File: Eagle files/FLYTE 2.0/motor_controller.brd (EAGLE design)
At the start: 160 x 100 mm, 21 parts, among them J1 XT60PW-F

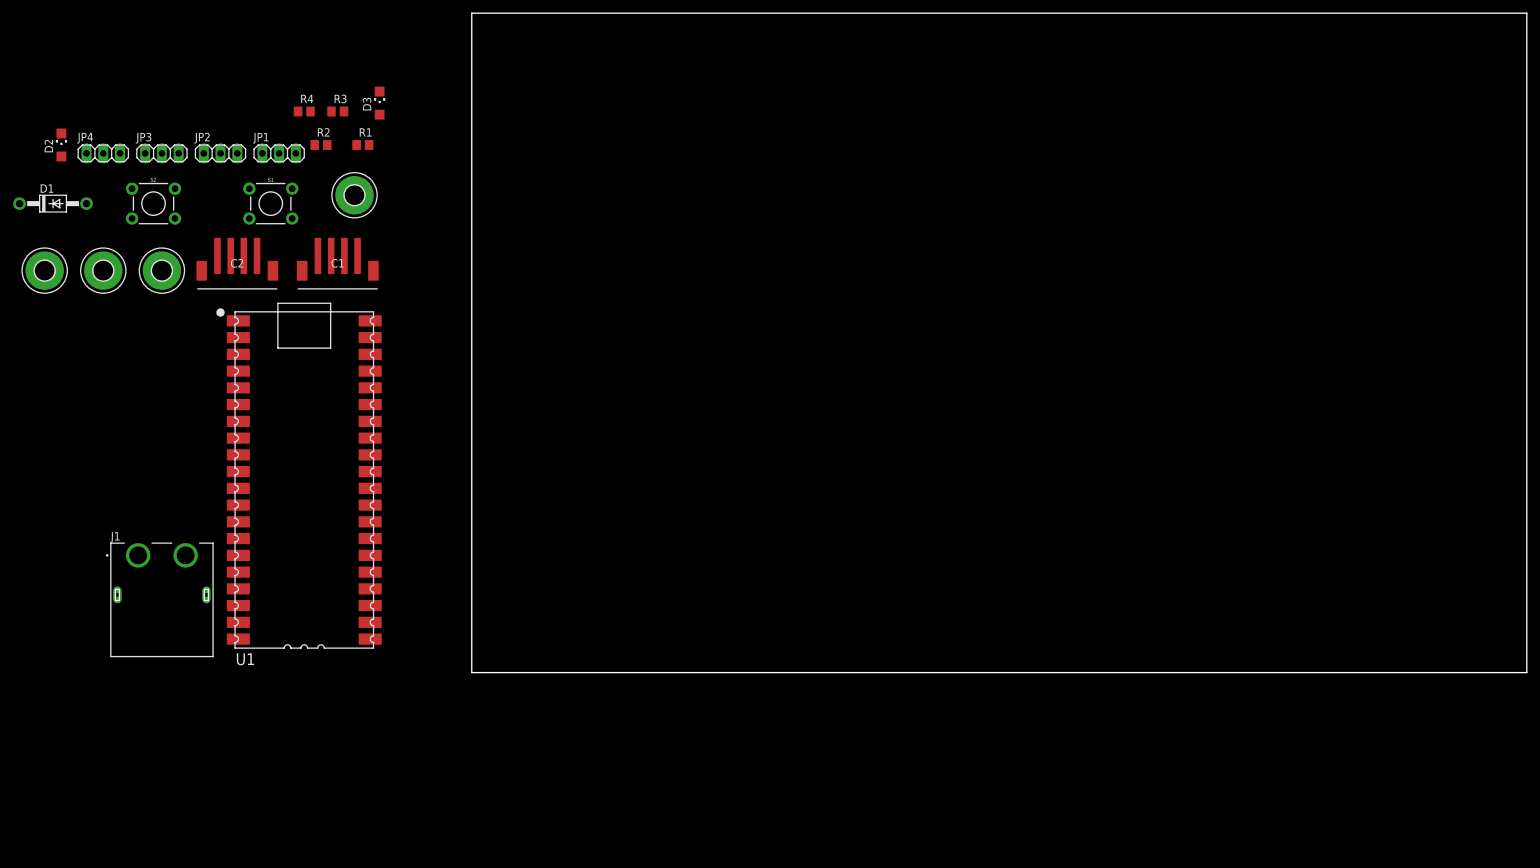
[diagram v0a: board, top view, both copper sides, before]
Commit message: Finish motor controller
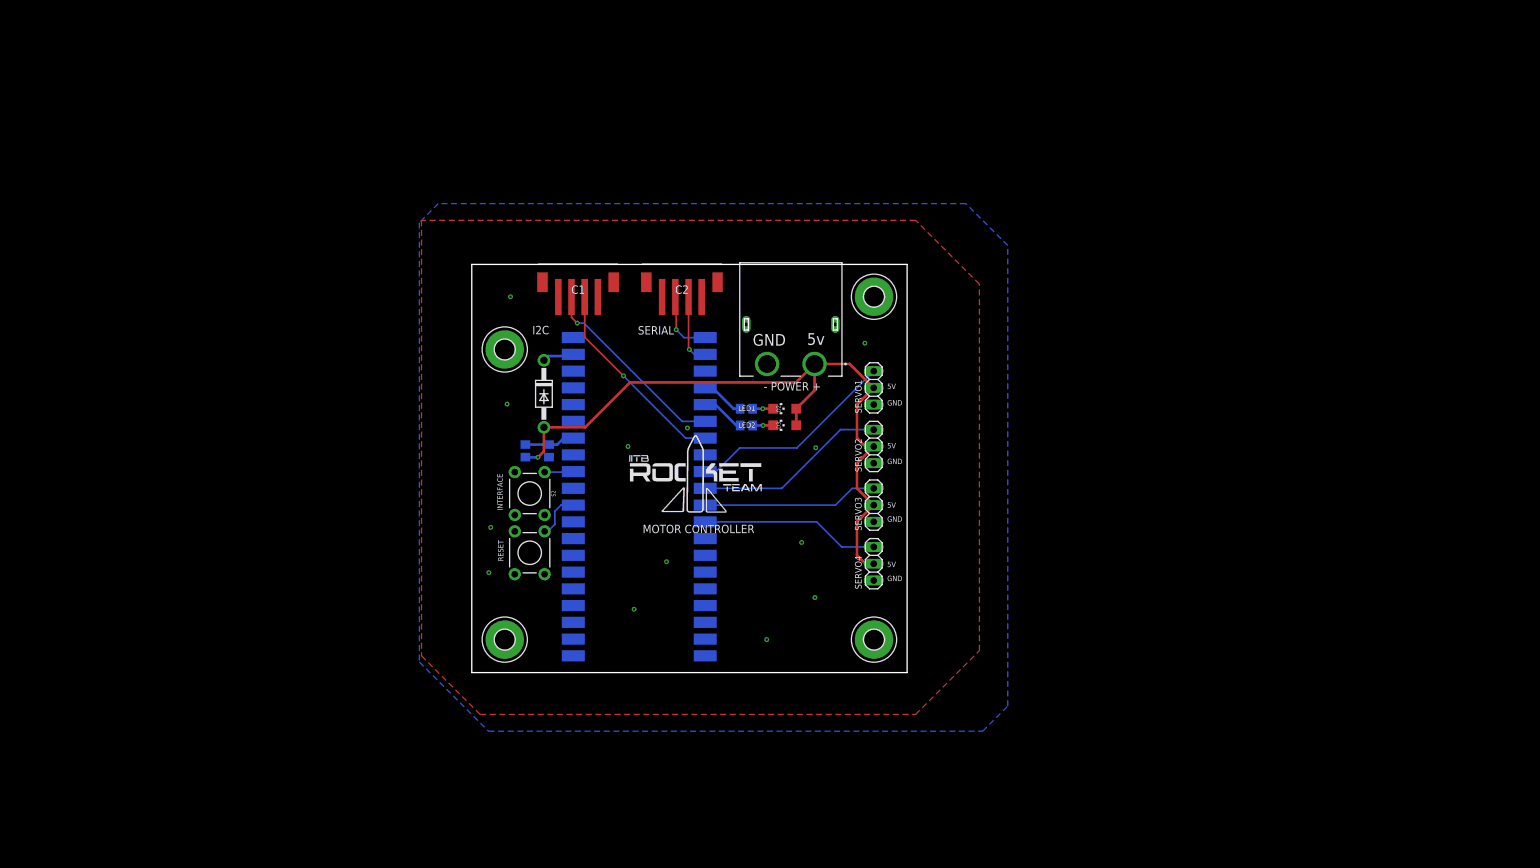
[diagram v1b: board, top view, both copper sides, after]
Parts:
- removed JP1, JP2, JP3, JP4: (no value), pinhead:1X03
- removed U1: (no value), RpiPico:PICO-PKG-NO_DEBUG
- added PICO: (no value), RpiPico:PICO-PKG-NO_DEBUG
- added SERVO1, SERVO2, SERVO3, SERVO4: (no value), pinhead:1X03
- moved H3 137.7 mm to (61.0, 5.00)
- moved D2 116.8 mm to (47.5, 40.0), turned to 90 degrees
- moved J1 99.7 mm to (48.4, 46.8), turned to 180 degrees
- moved H2 82.7 mm to (5.00, 5.00)
- moved R4 82.2 mm to (41.6, 37.5), flipped to the bottom, turned to 180 degrees
- moved H4 80.3 mm to (61.0, 57.0)
- moved D1 79.8 mm to (10.9, 42.3), turned to 270 degrees
- moved D3 78.5 mm to (47.5, 37.5), turned to 90 degrees
- moved R3 76.6 mm to (41.6, 40.0), flipped to the bottom, turned to 180 degrees
- moved S2 72.0 mm to (8.79, 27.2), turned to 270 degrees
- moved C2 67.4 mm to (31.9, 60.5), turned to 180 degrees
- moved S1 65.9 mm to (8.79, 18.2), turned to 270 degrees
- moved R2 55.8 mm to (8.13, 33.6), flipped to the bottom, turned to 90 degrees
- moved R1 54.3 mm to (11.7, 33.6), flipped to the bottom, turned to 90 degrees
- moved H1 53.3 mm to (5.00, 49.0)
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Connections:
- removed net N$7: D2.A, R3.1
- removed net N$8: D3.A, R4.1
- new net LED1: PICO.P$4, R3.1
- new net LED2: PICO.P$5, R4.1
- net 3V3(OUT): now also PICO.P$36; no longer U1.P$36
- net 5V: now also D2.A, D3.A, SERVO1.2, SERVO2.2, SERVO3.2, SERVO4.2; no longer JP1.2, JP2.2, JP3.2, JP4.2, R3.2, R4.2
- net GND: now also PICO.P$13, PICO.P$18, PICO.P$23, PICO.P$28, PICO.P$3, PICO.P$33, PICO.P$38, PICO.P$8, SERVO1.1, SERVO2.1, SERVO3.1, SERVO4.1; no longer JP1.1, JP2.1, JP3.1, JP4.1, U1.P$13, U1.P$18, U1.P$23, U1.P$28, U1.P$3, U1.P$33, U1.P$38, U1.P$8
- net N$1: now also PICO.P$39; no longer U1.P$39
- net N$2: now also PICO.P$30; no longer U1.P$30
- net N$3: now also PICO.P$32; no longer U1.P$32
- net N$4: now also PICO.P$34; no longer U1.P$34
- net N$5: now also R3.2; no longer U1.P$22
- net N$6: now also R4.2; no longer U1.P$21
- net SCL0: now also PICO.P$7; no longer U1.P$7
- net SDA0: now also PICO.P$6; no longer U1.P$6
- net SERVO1: now also PICO.P$9, SERVO1.3; no longer JP1.3, U1.P$9
- net SERVO2: now also PICO.P$10, SERVO2.3; no longer JP2.3, U1.P$10
- net SERVO3: now also PICO.P$11, SERVO3.3; no longer JP3.3, U1.P$11
- net SERVO4: now also PICO.P$12, SERVO4.3; no longer JP4.3, U1.P$12
- net SER_RX: now also PICO.P$2; no longer U1.P$2
- net SER_TX: now also PICO.P$1; no longer U1.P$1
- net VBUS: now also PICO.P$40; no longer U1.P$40
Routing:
- net 5V: track 0.00 -> 107.3 mm, vias 0 -> 1
- net SERVO1: track 0.00 -> 31.9 mm
- net SCL0: track 0.00 -> 30.7 mm, vias 0 -> 1
- net SDA0: track 0.00 -> 29.9 mm, vias 0 -> 1
- net SERVO2: track 0.00 -> 29.3 mm
- net SERVO4: track 0.00 -> 27.1 mm
- net SERVO3: track 0.00 -> 26.6 mm
- net SER_RX: track 0.00 -> 10.9 mm, vias 0 -> 1
- net SER_TX: track 0.00 -> 9.90 mm, vias 0 -> 1
- net N$4: track 0.00 -> 7.68 mm
- net N$2: track 0.00 -> 7.16 mm
- net LED1: track 0.00 -> 6.61 mm
- net LED2: track 0.00 -> 6.60 mm
- net N$1: track 0.00 -> 4.83 mm
- net N$3: track 0.00 -> 4.38 mm
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- added copper zone on layer 1, net GND
- added copper zone on layer 16, net GND
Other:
- board size 160 x 100 mm -> 66 x 61.9 mm
- board text added: "- POWER +"
- board text added: "5V"
- board text added: "5v"
- board text added: "GND"
- board text added: "I2C"
- board text added: "INTERFACE"
- board text added: "LED1"
- board text added: "LED2"
- board text added: "MOTOR CONTROLLER"
- board text added: "RESET"
- board text added: "SERIAL"

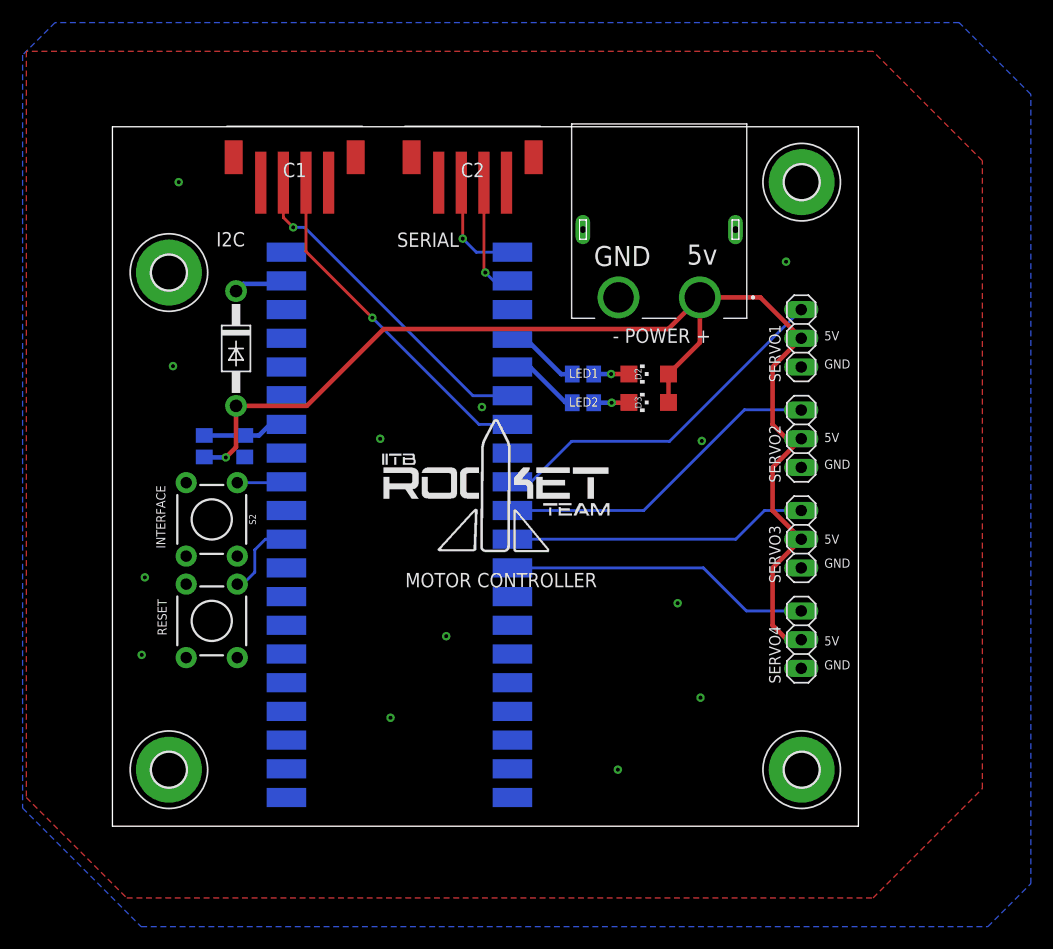
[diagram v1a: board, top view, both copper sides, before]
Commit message: minor changes
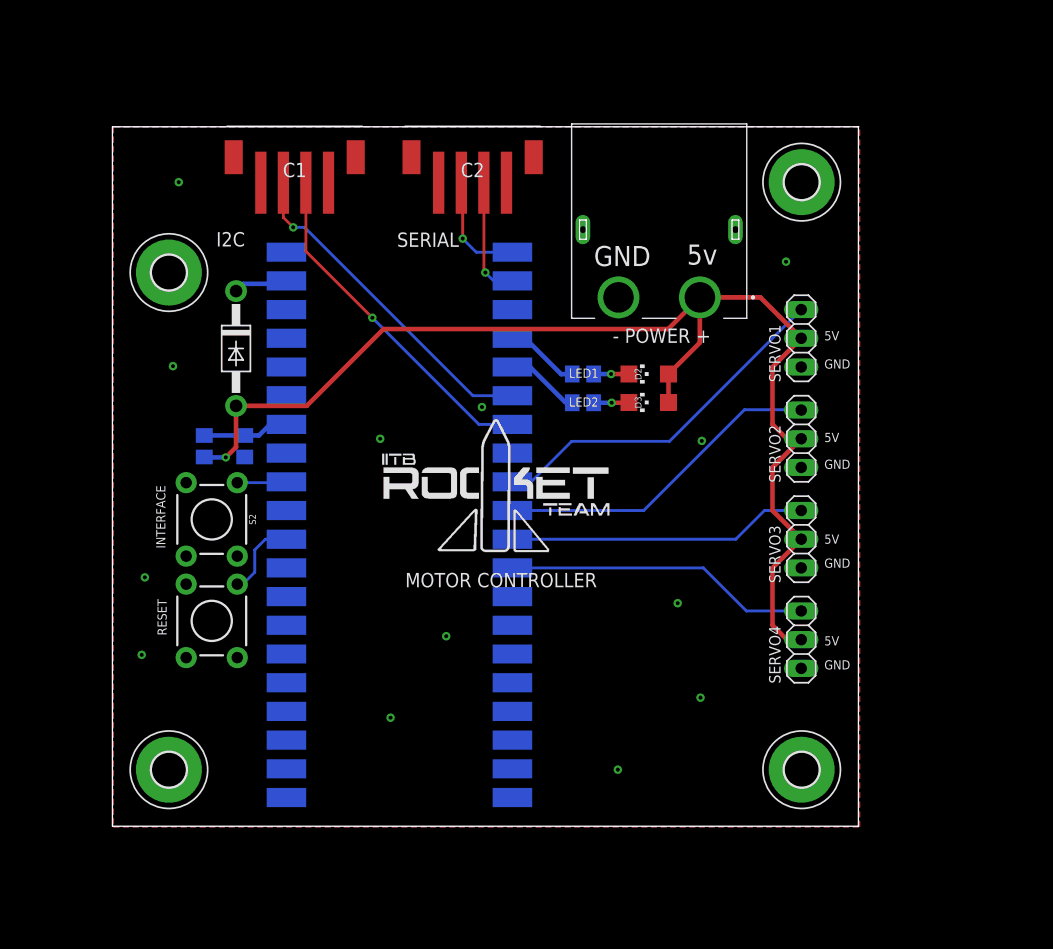
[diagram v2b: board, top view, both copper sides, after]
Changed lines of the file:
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@@
 <contactref element="R1" pad="1"/>
 <polygon width="0.254" layer="1">
-<vertex x="-7.62" y="68.58"/>
-<vertex x="-7.62" y="2.54"/>
-<vertex x="1.27" y="-6.35"/>
-<vertex x="67.31" y="-6.35"/>
-<vertex x="76.9874" y="3.3274"/>
-<vertex x="76.9874" y="58.9026"/>
-<vertex x="67.31" y="68.58"/>
+<vertex x="0.0762" y="61.9125"/>
+<vertex x="0.0762" y="-0.0635"/>
+<vertex x="66.1289" y="-0.0635"/>
+<vertex x="66.1289" y="61.9125"/>
 </polygon>
 <polygon width="0.254" layer="16">
-<vertex x="-7.9502" y="68.2498"/>
-<vertex x="-7.9502" y="1.6002"/>
-<vertex x="2.54" y="-8.89"/>
-<vertex x="77.47" y="-8.89"/>
-<vertex x="81.28" y="-5.08"/>
-<vertex x="81.28" y="64.77"/>
-<vertex x="74.93" y="71.12"/>
-<vertex x="-5.08" y="71.12"/>
+<vertex x="0.0889" y="61.8617"/>
+<vertex x="0.0889" y="-0.0508"/>
+<vertex x="66.0781" y="-0.0508"/>
+<vertex x="66.0781" y="61.8617"/>
 </polygon>
 <via x="5.8674" y="56.9976" extent="1-16" drill="0.35"/>

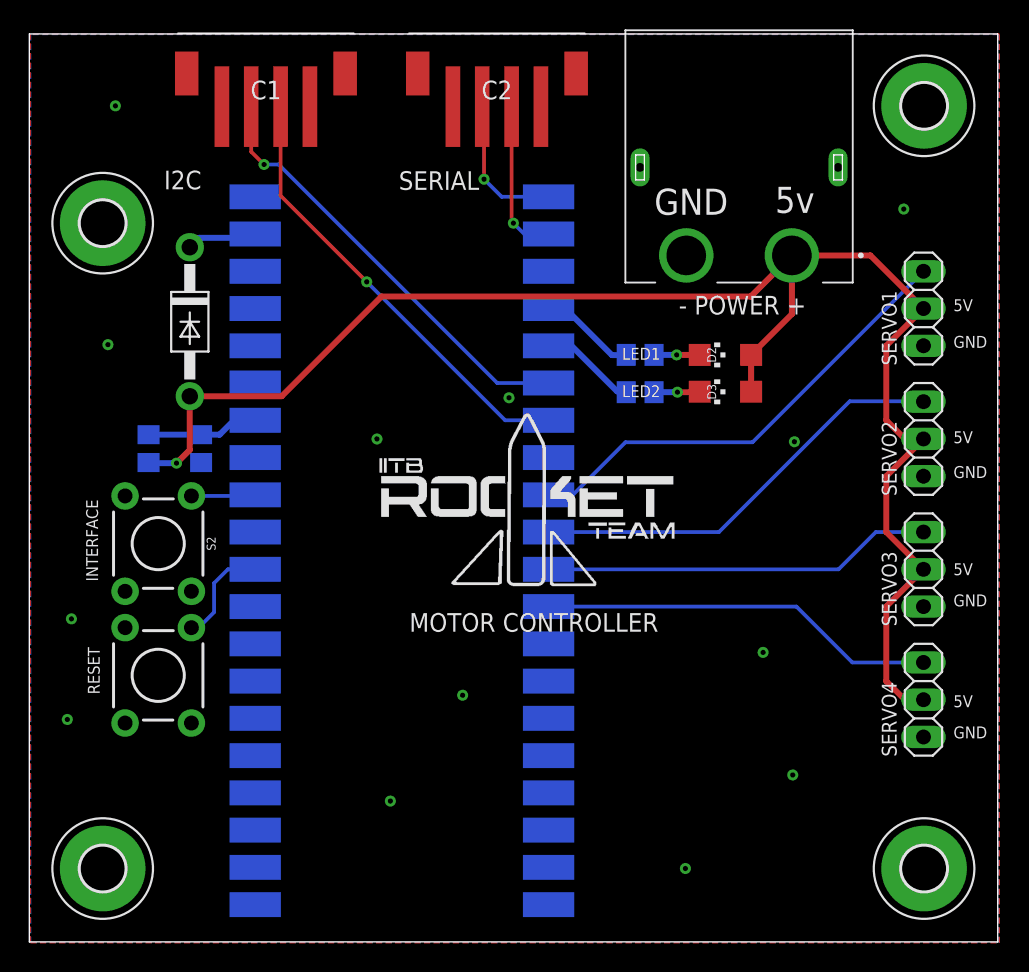
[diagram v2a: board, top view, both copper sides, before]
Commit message: Minor changes
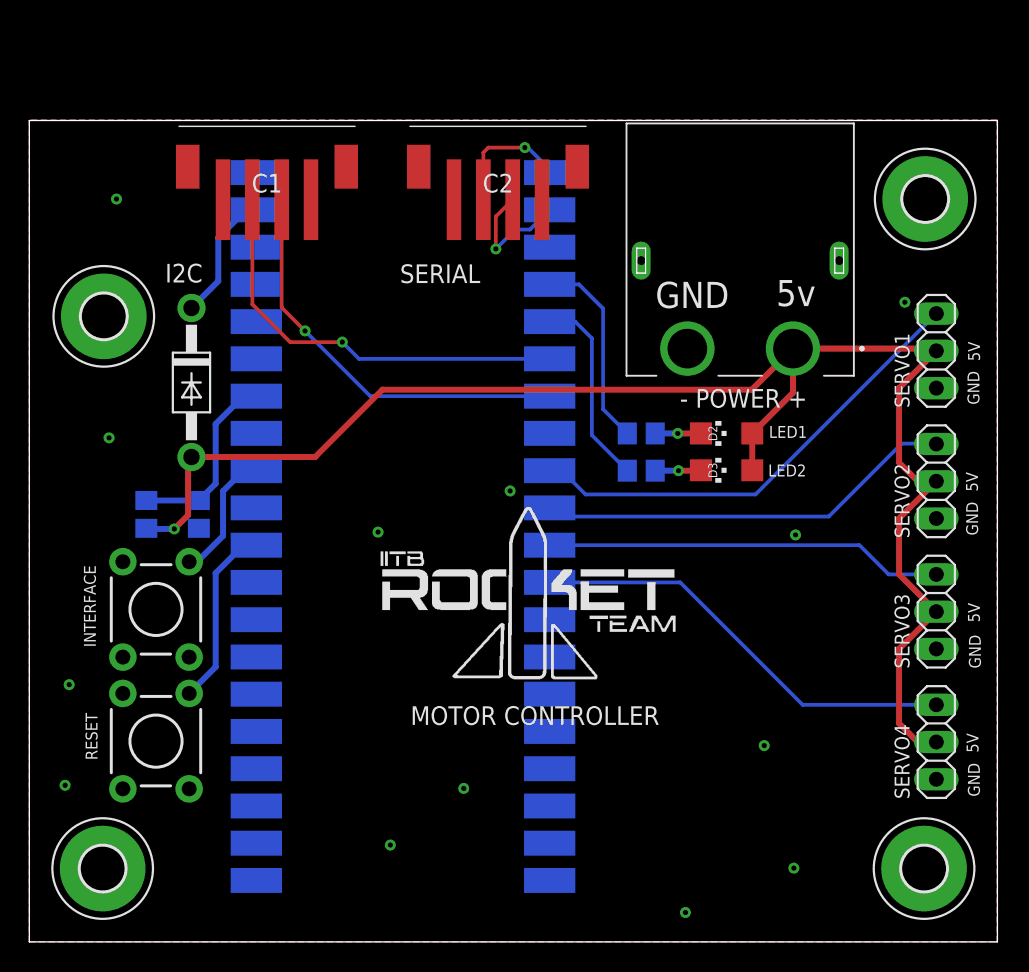
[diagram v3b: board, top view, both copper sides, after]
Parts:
- moved H1 6.35 mm to (5.08, 42.6)
- moved H4 6.35 mm to (61.1, 50.6)
- moved J1 6.35 mm to (48.5, 40.4)
- moved C1 6.35 mm to (16.2, 54.1)
- moved C2 6.35 mm to (32.0, 54.1)
- moved D3 5.35 mm to (47.5, 32.2)
- moved R4 5.35 mm to (41.7, 32.1)
- moved D2 5.35 mm to (47.5, 34.7)
- moved R3 5.35 mm to (41.7, 34.7)
- moved R1 4.49 mm to (11.6, 29.1)
- moved R2 4.49 mm to (7.98, 29.1)
- moved S1 4.49 mm to (8.64, 13.7)
- moved S2 4.49 mm to (8.64, 22.7)
- moved D1 4.14 mm to (11.1, 38.1)
- moved SERVO4 3.02 mm to (61.8, 13.6)
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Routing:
- net LED1: track 6.61 -> 13.5 mm
- net LED2: track 6.60 -> 13.4 mm
- net N$2: track 7.16 -> 12.5 mm
- net N$4: track 7.68 -> 12.8 mm
- net N$3: track 4.38 -> 8.94 mm
- net N$1: track 4.83 -> 8.92 mm
- net SERVO4: track 27.1 -> 29.8 mm
- net SCL0: track 30.7 -> 28.1 mm
- net SER_RX: track 10.9 -> 8.60 mm
- net 5V: track 107.3 -> 105.1 mm
- net SDA0: track 29.9 -> 28.9 mm
- net SER_TX: track 9.90 -> 9.00 mm
- net SERVO2: track 29.3 -> 28.7 mm
- net SERVO3: track 26.6 -> 27.2 mm
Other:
- board size 66 x 61.9 mm -> 66 x 56 mm
